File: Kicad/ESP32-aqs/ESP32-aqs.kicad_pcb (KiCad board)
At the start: 2 copper layers, 63.2 x 41.7 mm, 51 parts, among them IC1 CP2102N-A02-GQFN24, J1 USB4085-GF-A_REVA4, J2 JST connector SEN55, J3 ufl connector, J4 UART Connector, J6 test point / jst connector, Q1 IRLML0030, Q2 PMN48XP, Q3 SS8050-G, Q4 SS8050-G, SW1 TC-1102-B-C-B, SW2 TC-1102-B-C-B, U1 LD1117S33TR_SOT223, U2 ESP32-WROOM-32, U3 SGP41-D-R4, U4 SX1276S8S+T-X1

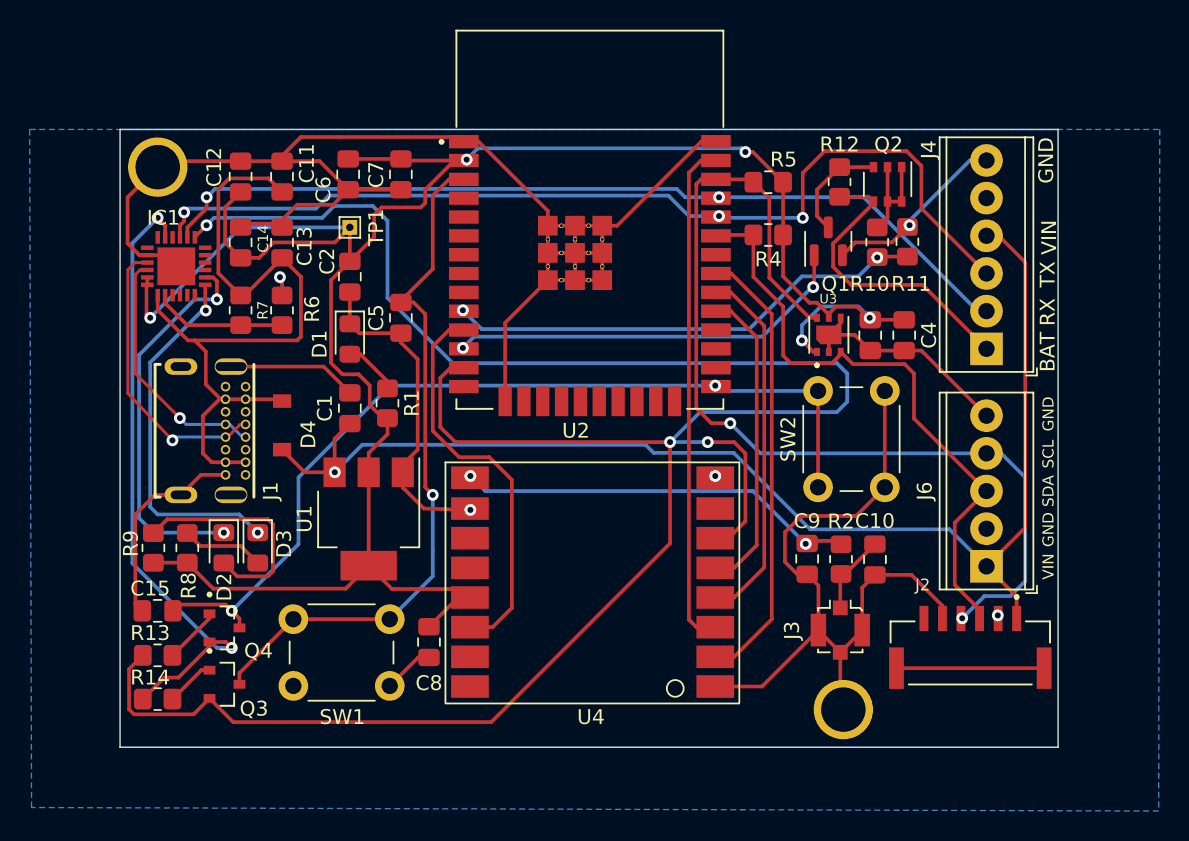
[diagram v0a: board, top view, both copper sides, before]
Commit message: PCB + BoM
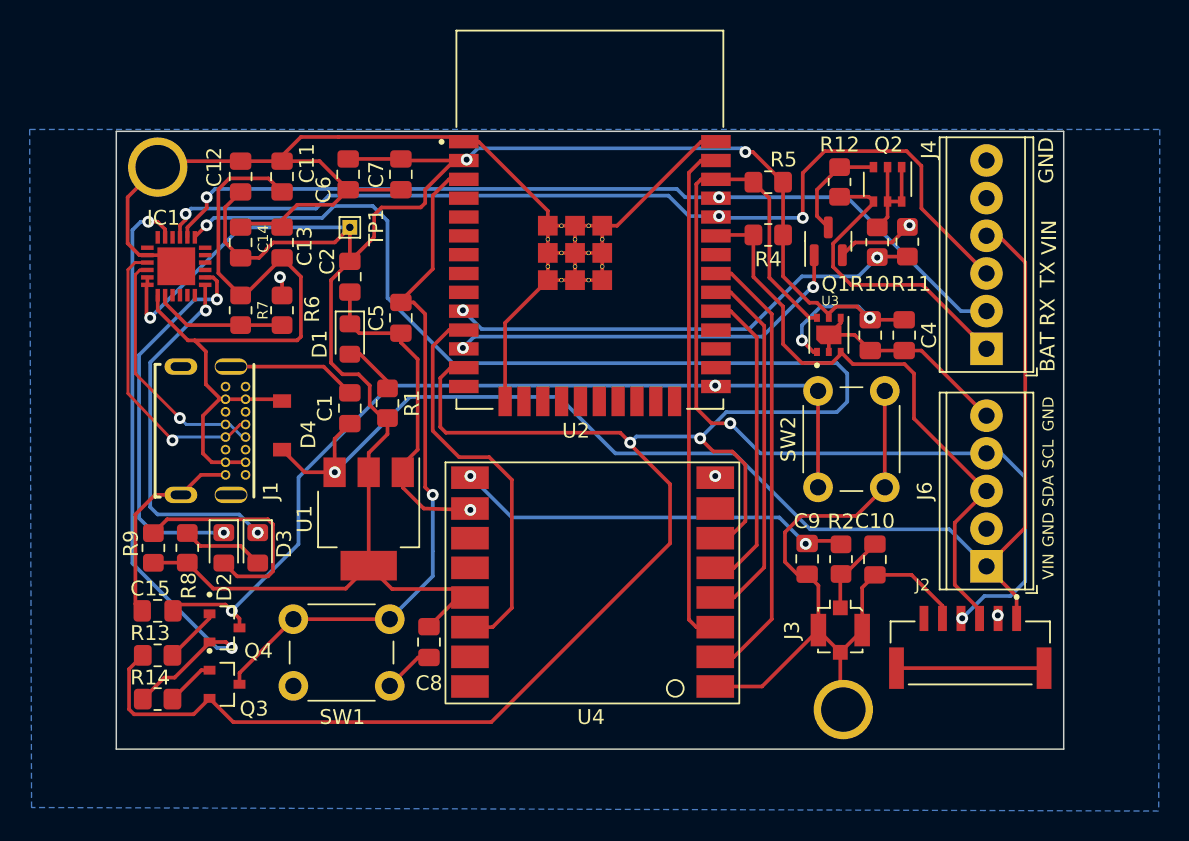
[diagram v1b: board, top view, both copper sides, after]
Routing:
- net GND: track 226.7 -> 219.5 mm
- net VIN: track 85.6 -> 88.3 mm
- net RST: track 154.9 -> 153.8 mm
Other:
- board size 63.2 x 41.7 mm -> 63.9 x 41.7 mm
